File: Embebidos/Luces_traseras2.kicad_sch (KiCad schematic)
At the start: 8 parts, among them J8 RJ45, Q5 BSS138, Q6 DMP3056LSDQ-13

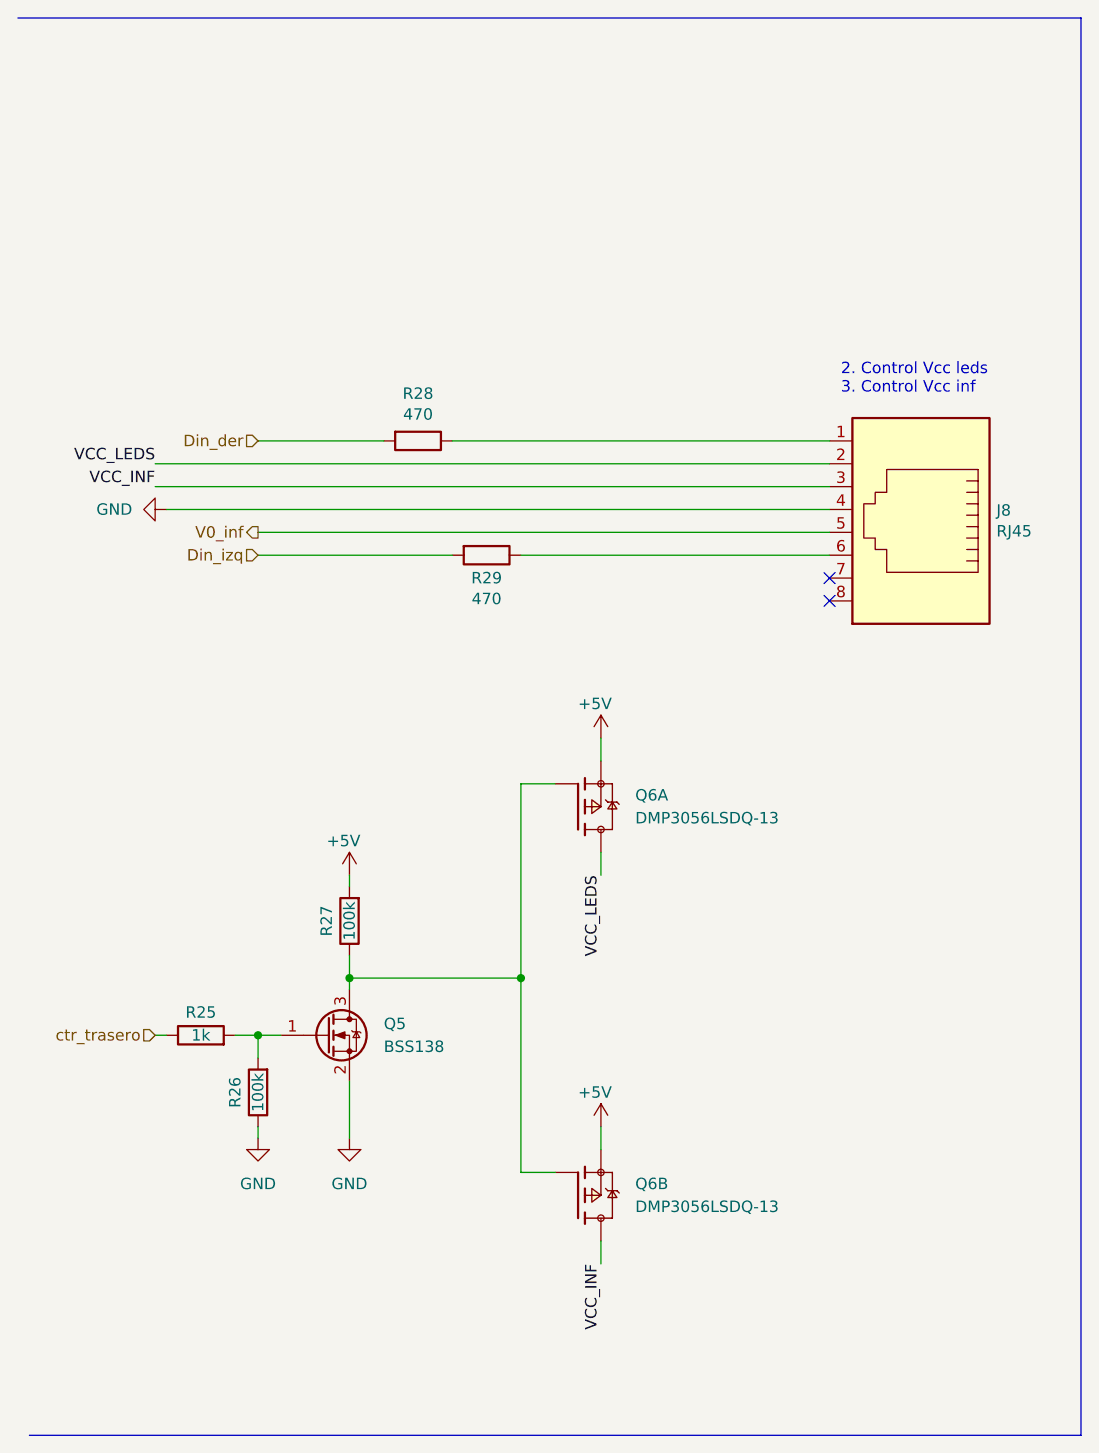
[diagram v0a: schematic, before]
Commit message: nosex2
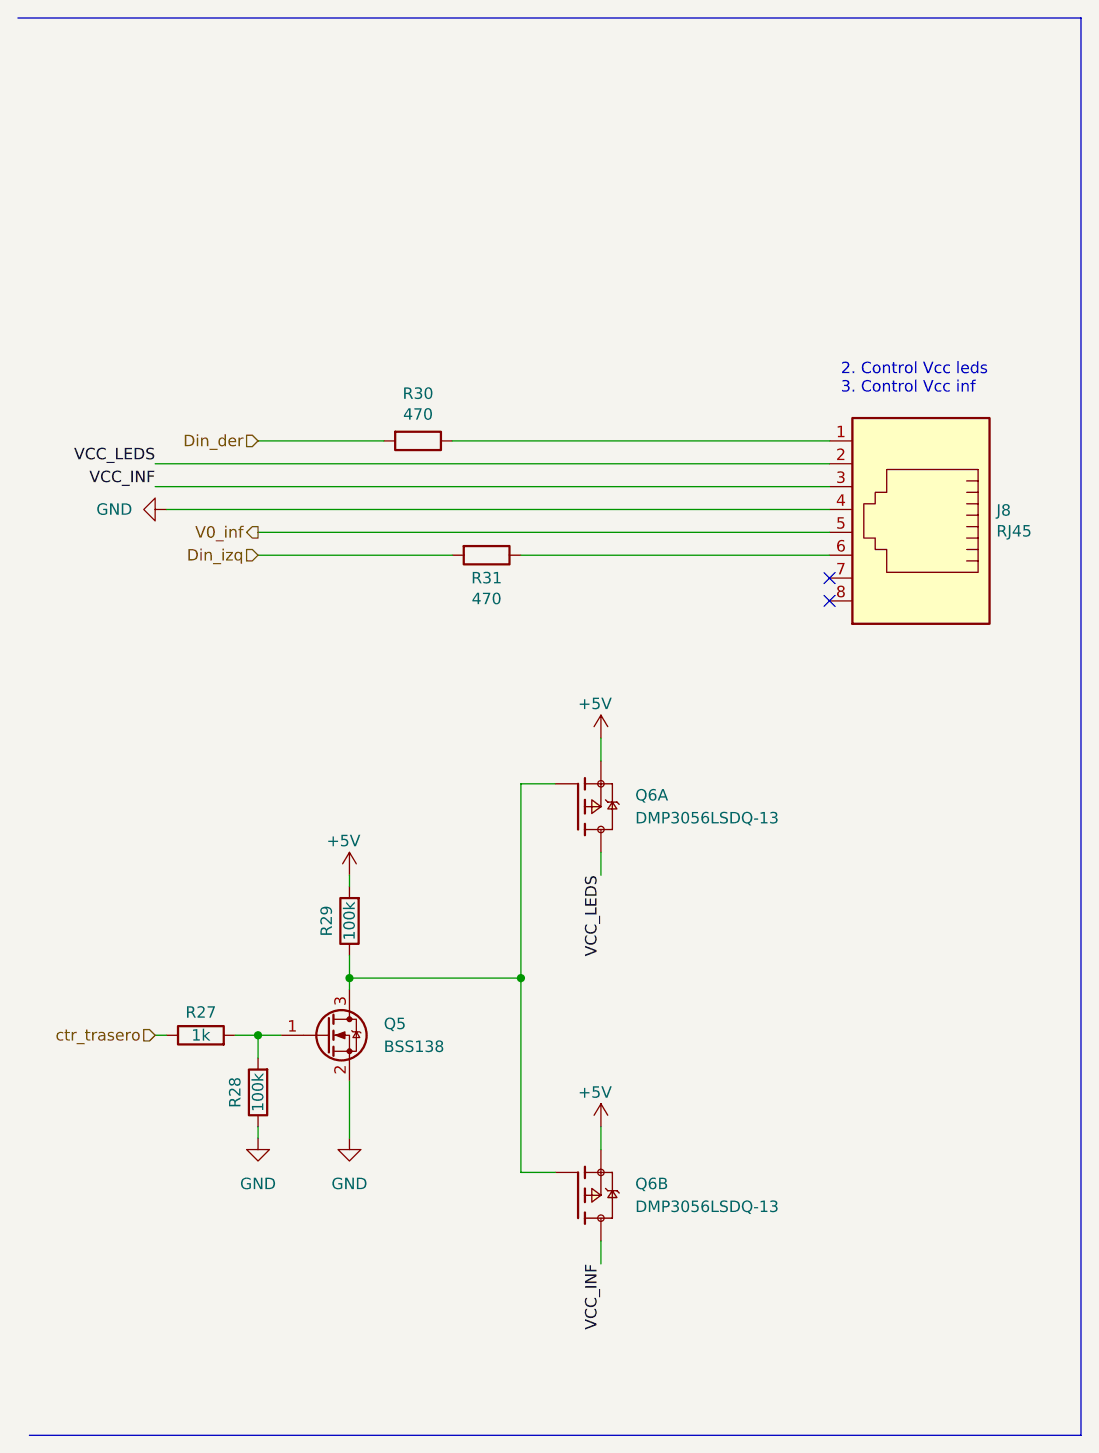
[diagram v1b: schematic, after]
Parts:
- renumbered R25 to R27, R26 to R28, R27 to R29, R28 to R30, R29 to R31
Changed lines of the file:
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@@
   (symbol (lib_id "Device:R") (at 55.88 83.82 270) (unit 1)
     (in_bom yes) (on_board yes)
-    (property "Reference" "R28" (id 0) (at 55.88 78.5622 90))
+    (property "Reference" "R30" (id 0) (at 55.88 78.5622 90))
     (property "Value" "470" (id 1) (at 55.88 80.8736 90))
     (property "Footprint" "" (id 2) (at 55.88 82.042 90)
@@
   (symbol (lib_id "Device:R") (at 63.5 96.52 270) (unit 1)
     (in_bom yes) (on_board yes)
-    (property "Reference" "R29" (id 0) (at 63.5 99.06 90))
+    (property "Reference" "R31" (id 0) (at 63.5 99.06 90))
     (property "Value" "470" (id 1) (at 63.5 101.3714 90))
     (property "Footprint" "" (id 2) (at 63.5 94.742 90)
@@
   (symbol (lib_id "Device:R") (at 31.75 149.86 90) (unit 1)
     (in_bom yes) (on_board yes)
-    (property "Reference" "R25" (id 0) (at 31.75 147.32 90))
+    (property "Reference" "R27" (id 0) (at 31.75 147.32 90))
     (property "Value" "1k" (id 1) (at 31.75 149.86 90))
     (property "Footprint" "" (id 2) (at 31.75 151.638 90)
@@
   (symbol (lib_id "Device:R") (at 48.26 137.16 180) (unit 1)
     (in_bom yes) (on_board yes)
-    (property "Reference" "R27" (id 0) (at 45.72 137.16 90))
+    (property "Reference" "R29" (id 0) (at 45.72 137.16 90))
     (property "Value" "100k" (id 1) (at 48.26 137.16 90))
     (property "Footprint" "" (id 2) (at 50.038 137.16 90)
@@
   (symbol (lib_id "Device:R") (at 38.1 156.21 180) (unit 1)
     (in_bom yes) (on_board yes)
-    (property "Reference" "R26" (id 0) (at 35.56 156.21 90))
+    (property "Reference" "R28" (id 0) (at 35.56 156.21 90))
     (property "Value" "100k" (id 1) (at 38.1 156.21 90))
     (property "Footprint" "" (id 2) (at 39.878 156.21 90)

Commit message: r33
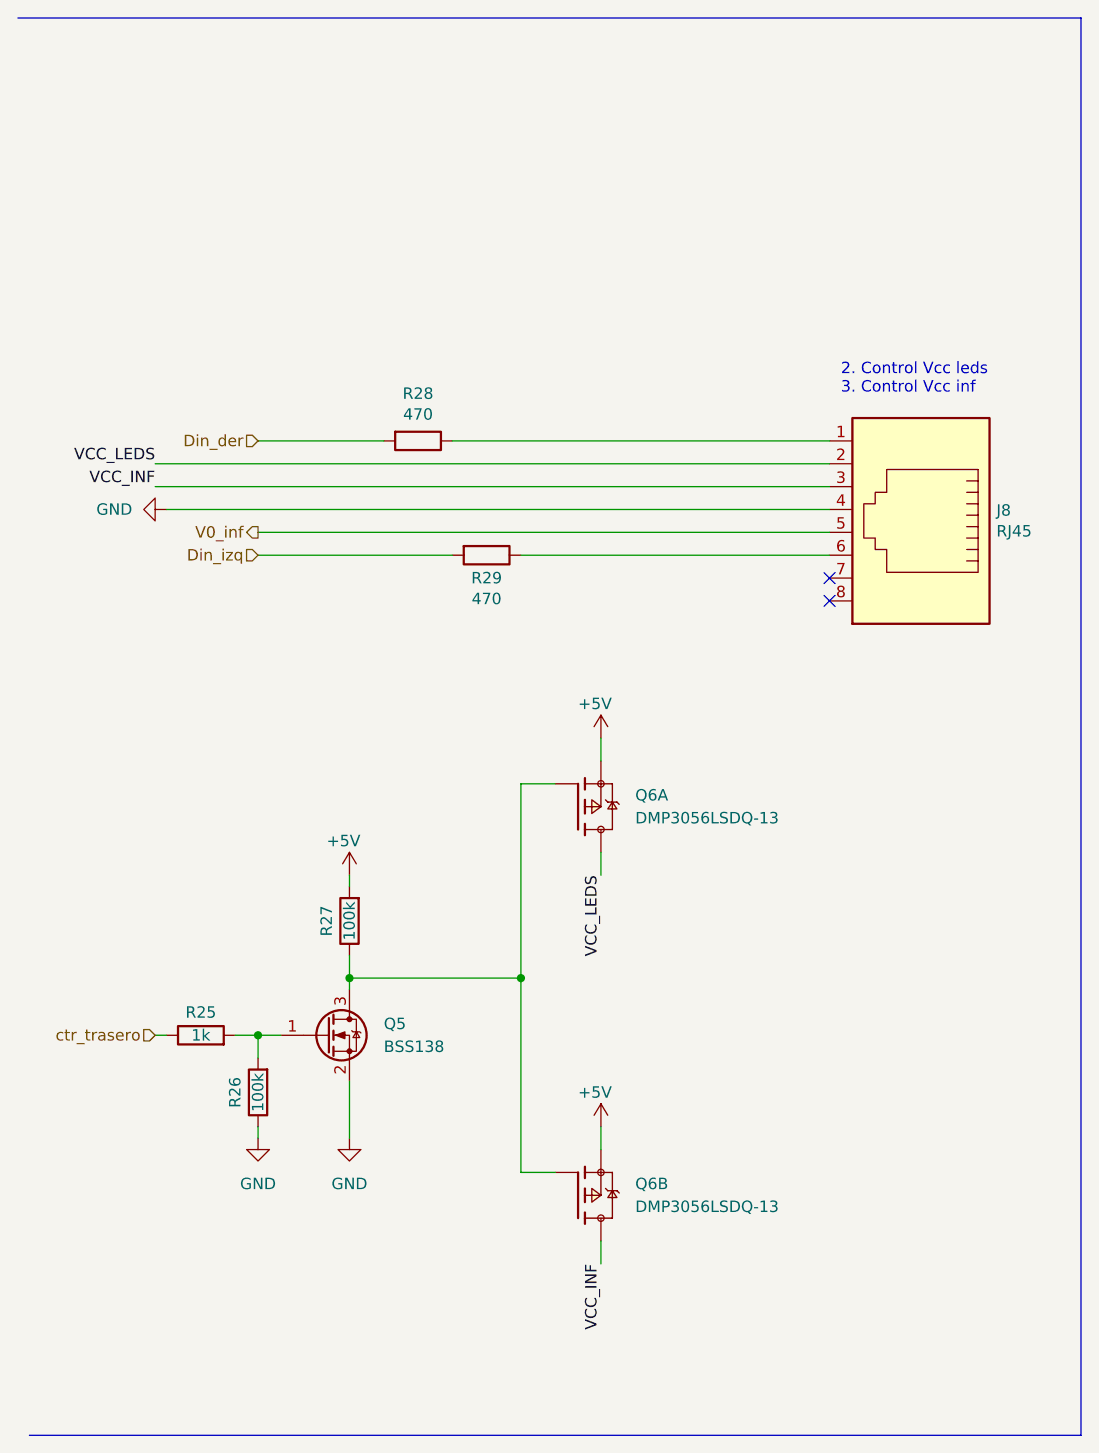
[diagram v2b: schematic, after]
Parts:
- renumbered R27 to R25, R28 to R26, R29 to R27, R30 to R28, R31 to R29
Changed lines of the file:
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@@
   (symbol (lib_id "Device:R") (at 55.88 83.82 270) (unit 1)
     (in_bom yes) (on_board yes)
-    (property "Reference" "R30" (id 0) (at 55.88 78.5622 90))
+    (property "Reference" "R28" (id 0) (at 55.88 78.5622 90))
     (property "Value" "470" (id 1) (at 55.88 80.8736 90))
     (property "Footprint" "" (id 2) (at 55.88 82.042 90)
@@
   (symbol (lib_id "Device:R") (at 63.5 96.52 270) (unit 1)
     (in_bom yes) (on_board yes)
-    (property "Reference" "R31" (id 0) (at 63.5 99.06 90))
+    (property "Reference" "R29" (id 0) (at 63.5 99.06 90))
     (property "Value" "470" (id 1) (at 63.5 101.3714 90))
     (property "Footprint" "" (id 2) (at 63.5 94.742 90)
@@
   (symbol (lib_id "Device:R") (at 31.75 149.86 90) (unit 1)
     (in_bom yes) (on_board yes)
-    (property "Reference" "R27" (id 0) (at 31.75 147.32 90))
+    (property "Reference" "R25" (id 0) (at 31.75 147.32 90))
     (property "Value" "1k" (id 1) (at 31.75 149.86 90))
     (property "Footprint" "" (id 2) (at 31.75 151.638 90)
@@
   (symbol (lib_id "Device:R") (at 48.26 137.16 180) (unit 1)
     (in_bom yes) (on_board yes)
-    (property "Reference" "R29" (id 0) (at 45.72 137.16 90))
+    (property "Reference" "R27" (id 0) (at 45.72 137.16 90))
     (property "Value" "100k" (id 1) (at 48.26 137.16 90))
     (property "Footprint" "" (id 2) (at 50.038 137.16 90)
@@
   (symbol (lib_id "Device:R") (at 38.1 156.21 180) (unit 1)
     (in_bom yes) (on_board yes)
-    (property "Reference" "R28" (id 0) (at 35.56 156.21 90))
+    (property "Reference" "R26" (id 0) (at 35.56 156.21 90))
     (property "Value" "100k" (id 1) (at 38.1 156.21 90))
     (property "Footprint" "" (id 2) (at 39.878 156.21 90)
